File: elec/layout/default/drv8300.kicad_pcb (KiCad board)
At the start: 2 copper layers, 225.7 x 100.8 mm, 0 parts

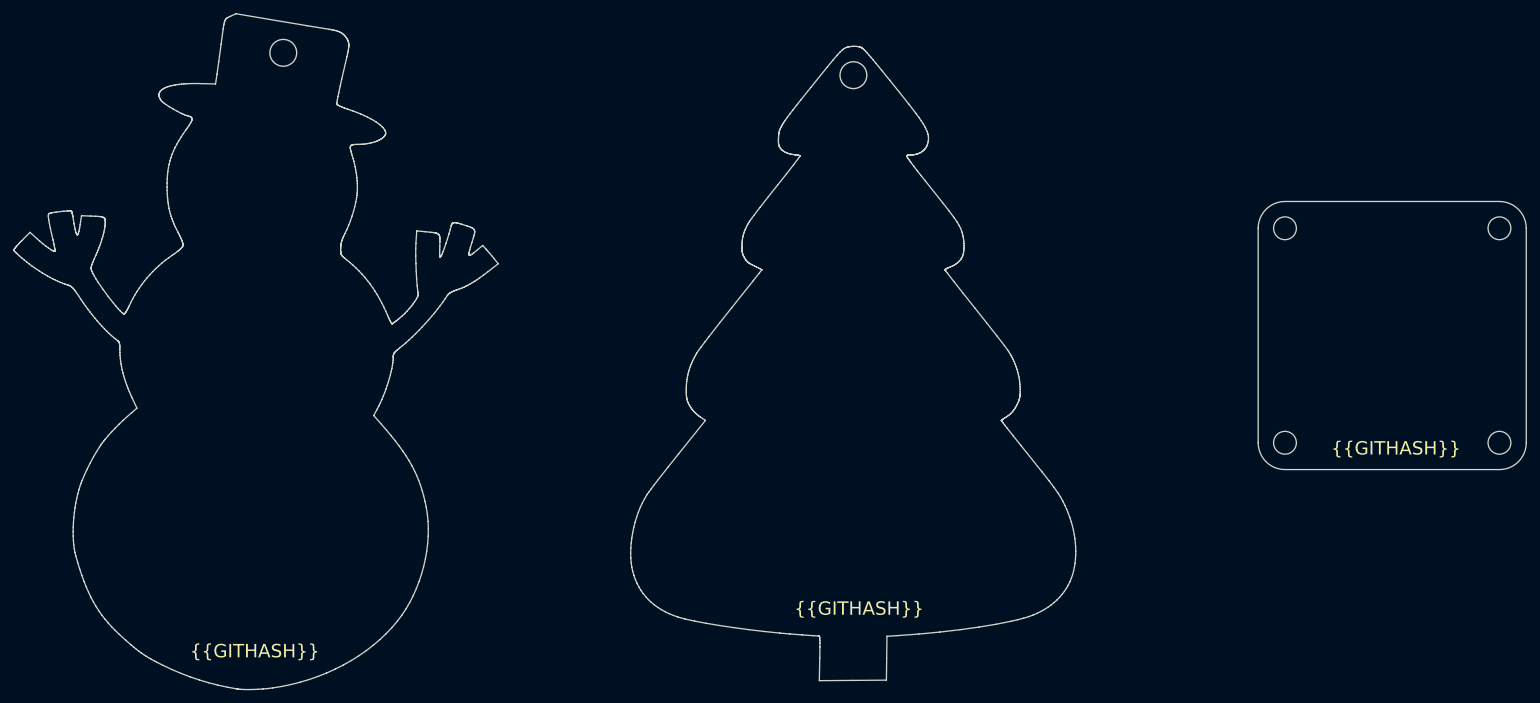
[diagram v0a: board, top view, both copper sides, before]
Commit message: initial build - has bugs
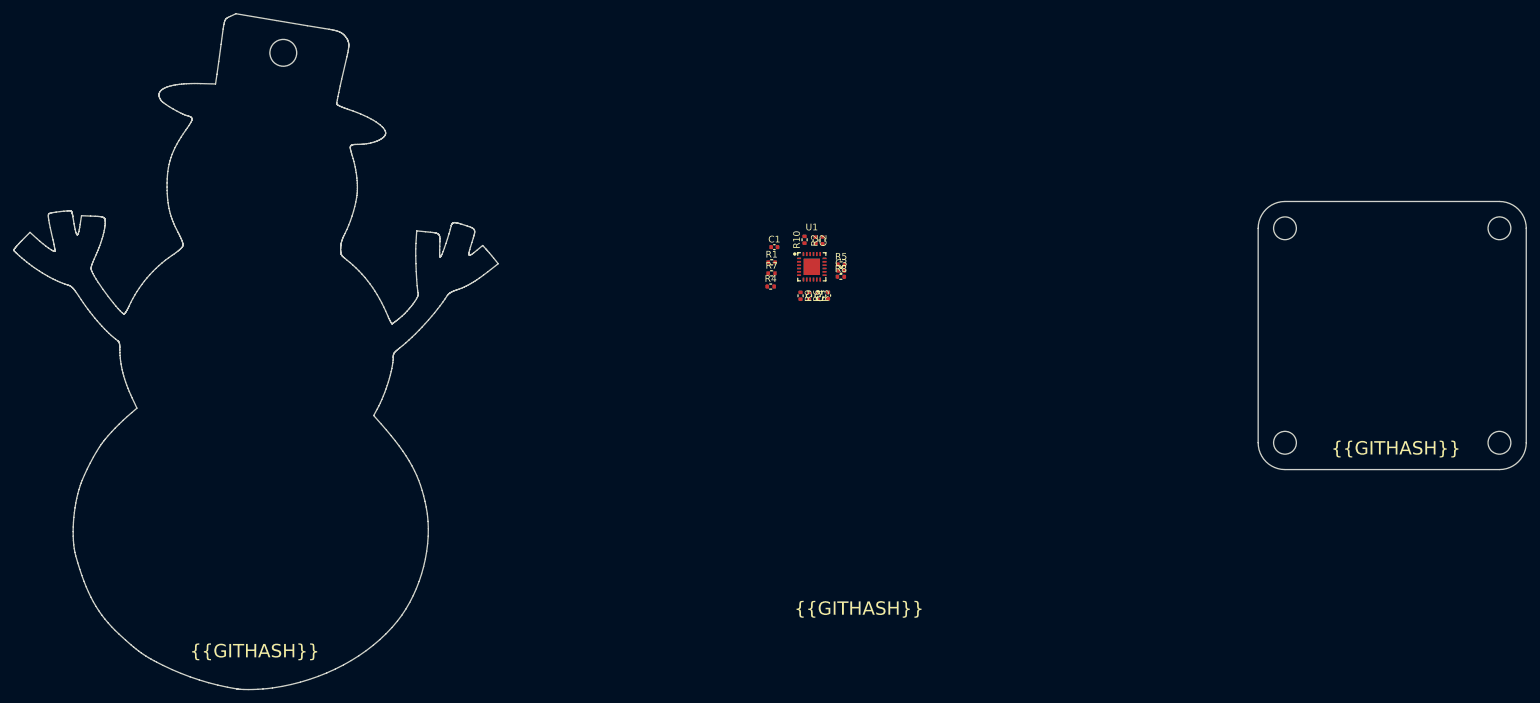
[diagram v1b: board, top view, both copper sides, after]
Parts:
- added C1: 25V 1uF X5R ±10% 0402 Multilayer Ceramic Capacitors MLCC - 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, lib:C0402, F.Cu at (149.4, 84.6)
- added C2: 25V 1uF X5R ±10% 0402 Multilayer Ceramic Capacitors MLCC - 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, lib:C0402, F.Cu at (155.6, 83.6)
- added C3: 25V 1uF X5R ±10% 0402 Multilayer Ceramic Capacitors MLCC - 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, lib:C0402, F.Cu at (159.4, 88.1)
- added C4: 25V 1uF X5R ±10% 0402 Multilayer Ceramic Capacitors MLCC - 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, lib:C0402, F.Cu at (157.5, 91.8)
- added R1: Chip Resistor - Surface Mount 4.7KOhms ±5% 1/16W 0402 RoHS, lib:R0402, F.Cu at (149.0, 86.9)
- added R10: Chip Resistor - Surface Mount 39KOhms ±5% 1/16W 0402 RoHS, lib:R0402, F.Cu at (153.9, 83.5)
- added R2: Chip Resistor - Surface Mount 10Ohms ±5% 1/16W 0402 RoHS, lib:R0402, F.Cu at (156.6, 83.6)
- added R3: Chip Resistor - Surface Mount 10Ohms ±5% 1/16W 0402 RoHS, lib:R0402, F.Cu at (155.9, 91.8)
- added R4: Chip Resistor - Surface Mount 4.7KOhms ±5% 1/16W 0402 RoHS, lib:R0402, F.Cu at (148.9, 90.5)
- added R5: Chip Resistor - Surface Mount 10Ohms ±5% 1/16W 0402 RoHS, lib:R0402, F.Cu at (159.4, 87.2)
- added R6: Chip Resistor - Surface Mount 10Ohms ±5% 1/16W 0402 RoHS, lib:R0402, F.Cu at (154.6, 91.8)
- added R7: Chip Resistor - Surface Mount 4.7KOhms ±5% 1/16W 0402 RoHS, lib:R0402, F.Cu at (149.0, 88.5)
- added R8: Chip Resistor - Surface Mount 10Ohms ±5% 1/16W 0402 RoHS, lib:R0402, F.Cu at (159.4, 89.0)
- added R9: Chip Resistor - Surface Mount 10Ohms ±5% 1/16W 0402 RoHS, lib:R0402, F.Cu at (153.3, 91.9)
- added U1: , lib:VQFN-24_L4.0-W4.0-P0.50-TL-EP2.5, F.Cu at (155.0, 87.5)
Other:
- outline, holes or cut-outs redrawn
